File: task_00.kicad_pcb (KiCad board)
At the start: 2 copper layers, 36.2 x 31.1 mm, 30 parts, among them J1 Screw_Terminal_01x02, 3935700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, J2 Screw_Terminal_01x02, 3935700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, Q1 FQP27P06, U1 TPS54360DDAR

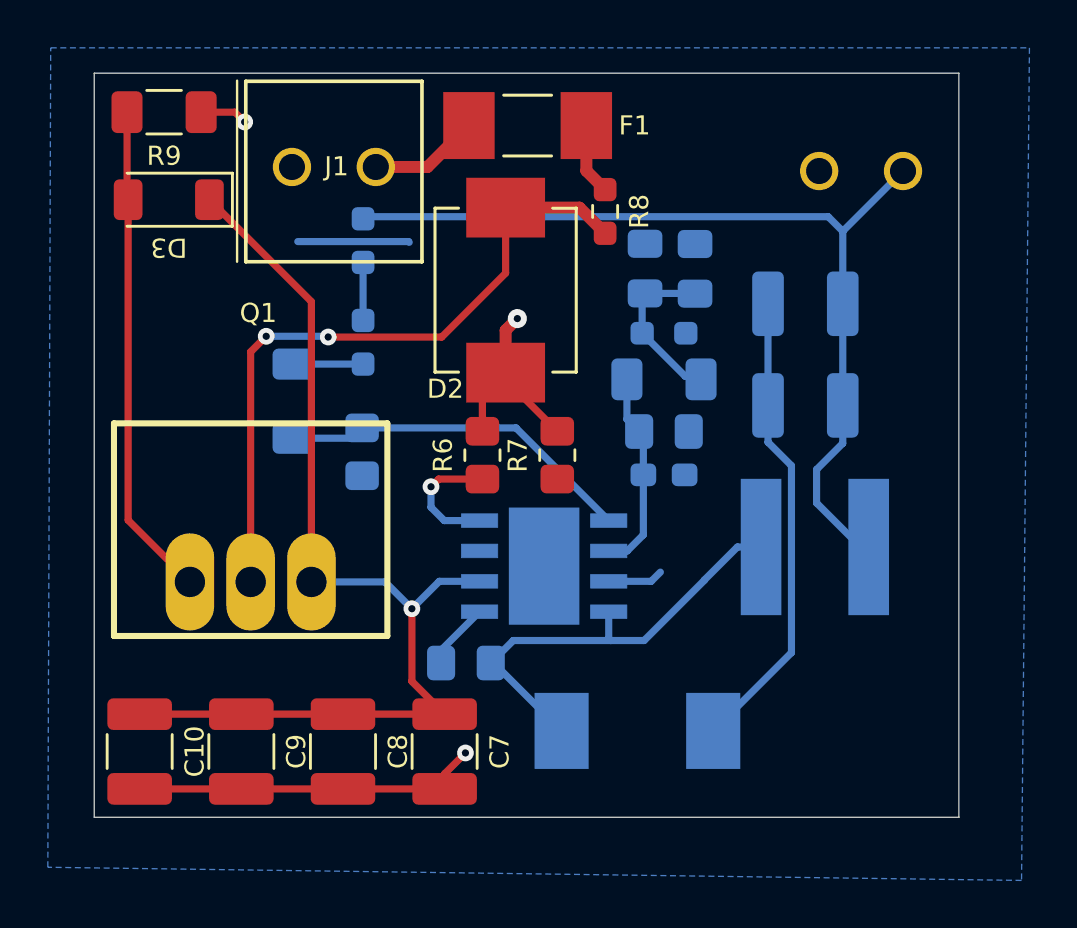
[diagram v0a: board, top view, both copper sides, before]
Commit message: Finished with version 0 of the proj
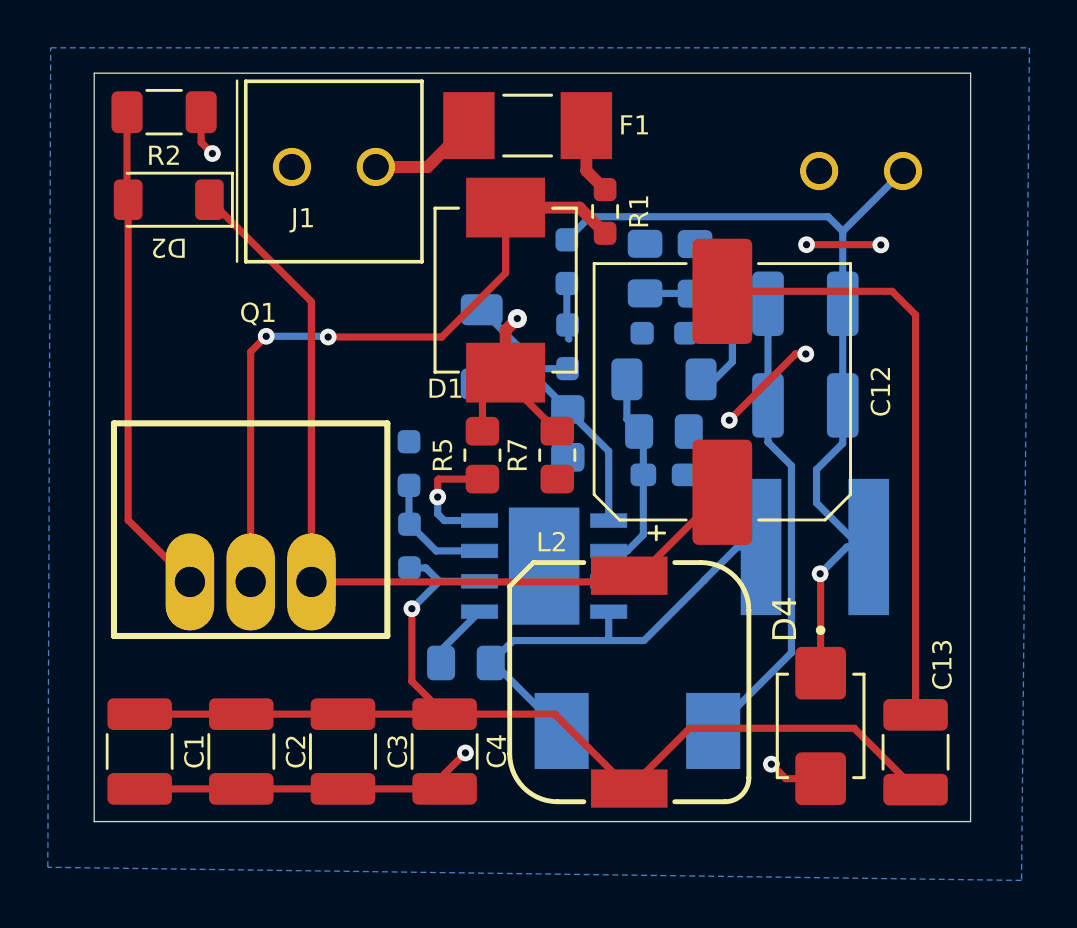
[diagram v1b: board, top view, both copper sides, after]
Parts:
- added C12: 47uF, EFVL100ADA470M10B0, Capacitor_SMD:CP_Elec_10x10.5, F.Cu at (117.3, 90.4)
- added C13: 10uF, C3225X7R2A106K250AC, Capacitor_SMD:C_1210_3225Metric_Pad1.33x2.70mm_HandSolder, F.Cu at (125.4, 105.4)
- added D4: SMLVT3V3, SMLVT3V3:DIOM5336X265N, F.Cu at (121.4, 104.3)
- added L2: CDRH104R, CDRH104R:CDRH104R, F.Cu at (113.4, 102.5)
- added R3: 253k, 0603WAF5233T5E, Resistor_SMD:R_0603_1608Metric_Pad0.98x0.95mm_HandSolder, B.Cu at (104.2, 96.8)
- added R4: 84.5k, 0603WAF8452T5E, Resistor_SMD:R_0603_1608Metric_Pad0.98x0.95mm_HandSolder, B.Cu at (104.2, 93.4)
- moved R10 8.63 mm to (110.8, 92.1)
- moved R7 8.57 mm to (110.8, 84.9)
- moved R8 8.55 mm to (110.8, 88.5)
- moved R9 8.19 mm to (107.2, 88.5)
- renumbered C10 to C1, C3 to C10, C9 to C2, C8 to C3, C7 to C4, C1 to C5, C4 to C6, C5 to C7, C2 to C8, C6 to C9, D2 to D1, D3 to D2, D1 to D3, R8 to R1, R1 to R10, R9 to R2, R6 to R5, R3 to R6, R2 to R7, R5 to R8, R7 to R9
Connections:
- C1 pad 1: Net-(D3-K) (its old number) -> /VIN
- C2 pad 1: Net-(D3-K) (its old number) -> /VIN
- C3 pad 1: Net-(D3-K) (its old number) -> /VIN
- C4 pad 1: Net-(D3-K) (its old number) -> /VIN
- C6 pad 1: Net-(C4-Pad1) -> Net-(C6-Pad1)
- C7 pad 1: Net-(C4-Pad1) -> Net-(C6-Pad1)
- D2 pad 1: Net-(D3-K) (its old number) -> /VIN_sp
- Q1 pad 3: Net-(D3-K) (its old number) -> /VIN_sp
- R6 pad 2: Net-(C4-Pad1) -> Net-(C6-Pad1)
- U1 pad 2: Net-(D3-K) (its old number) -> /VIN
- U1 pad 3: unconnected-(U1-EN-Pad3) -> /EN
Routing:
- net /VIN: track 0.00 -> 45.6 mm, vias 0 -> 1
- net Net-(D3-K) (its old number): track 43.4 -> 0.00 mm, vias 1 -> 0
- net /VIN_sp: track 0.00 -> 36.5 mm
- net Net-(C12-Pad2): track 0.00 -> 25.2 mm
- net Net-(C6-Pad1): track 0.00 -> 7.34 mm
- net Net-(C4-Pad1): track 7.29 -> 0.14 mm
- net /FB: track 15.0 -> 9.48 mm
- net /EN: track 0.00 -> 5.04 mm
- net GND: track 32.8 -> 37.8 mm, vias 3 -> 8
- net Net-(R8-Pad2): track 2.91 -> 4.61 mm
- net /V_OUT: track 38.3 -> 36.9 mm, vias 0 -> 1
- net Net-(R7-Pad2): track 2.31 -> 1.75 mm
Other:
- board size 36.2 x 31.1 mm -> 36.6 x 31.3 mm
